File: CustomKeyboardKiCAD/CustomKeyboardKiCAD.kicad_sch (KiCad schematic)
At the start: 4 parts, among them J1 USB_C_Receptacle_USB2.0_16P, U1 nRF52840

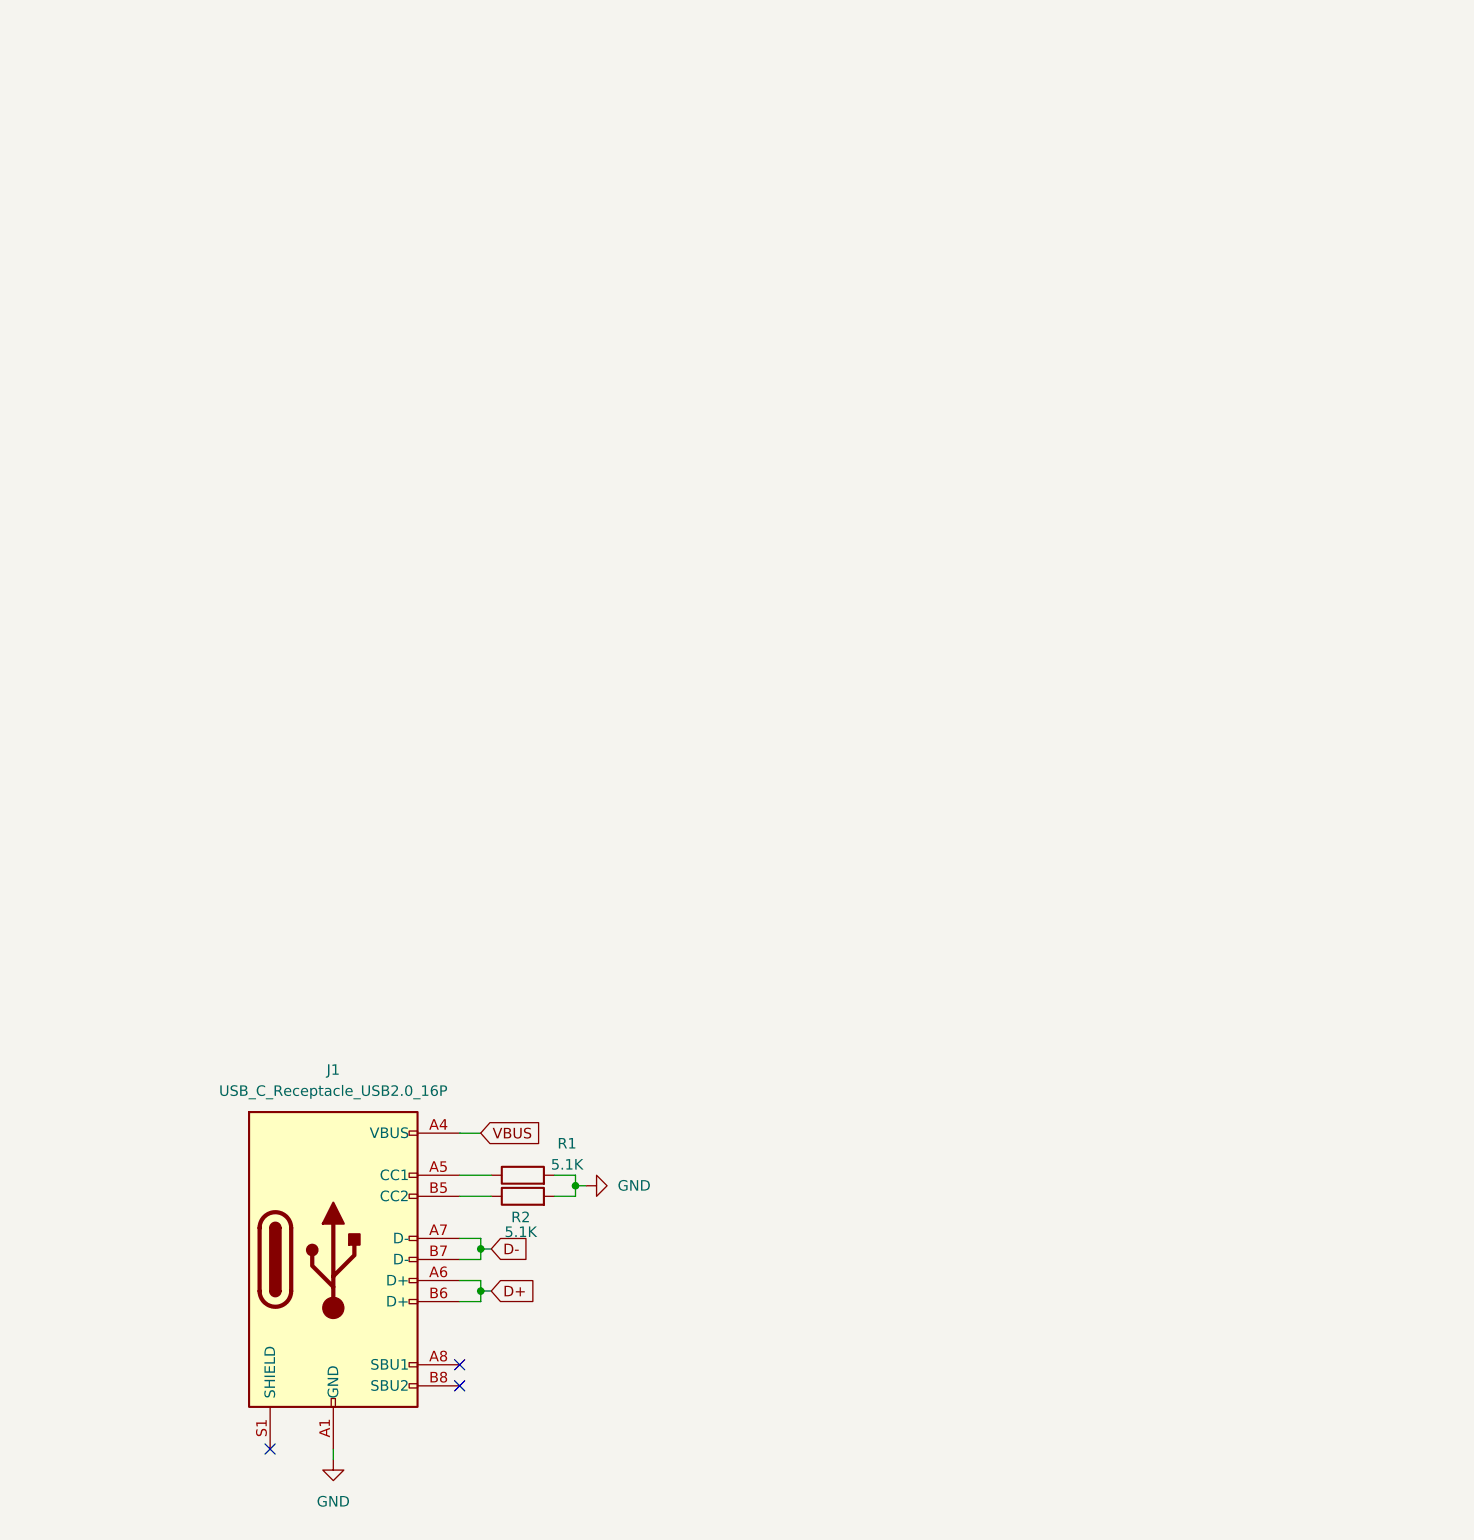
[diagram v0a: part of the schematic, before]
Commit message: Progress on schematic
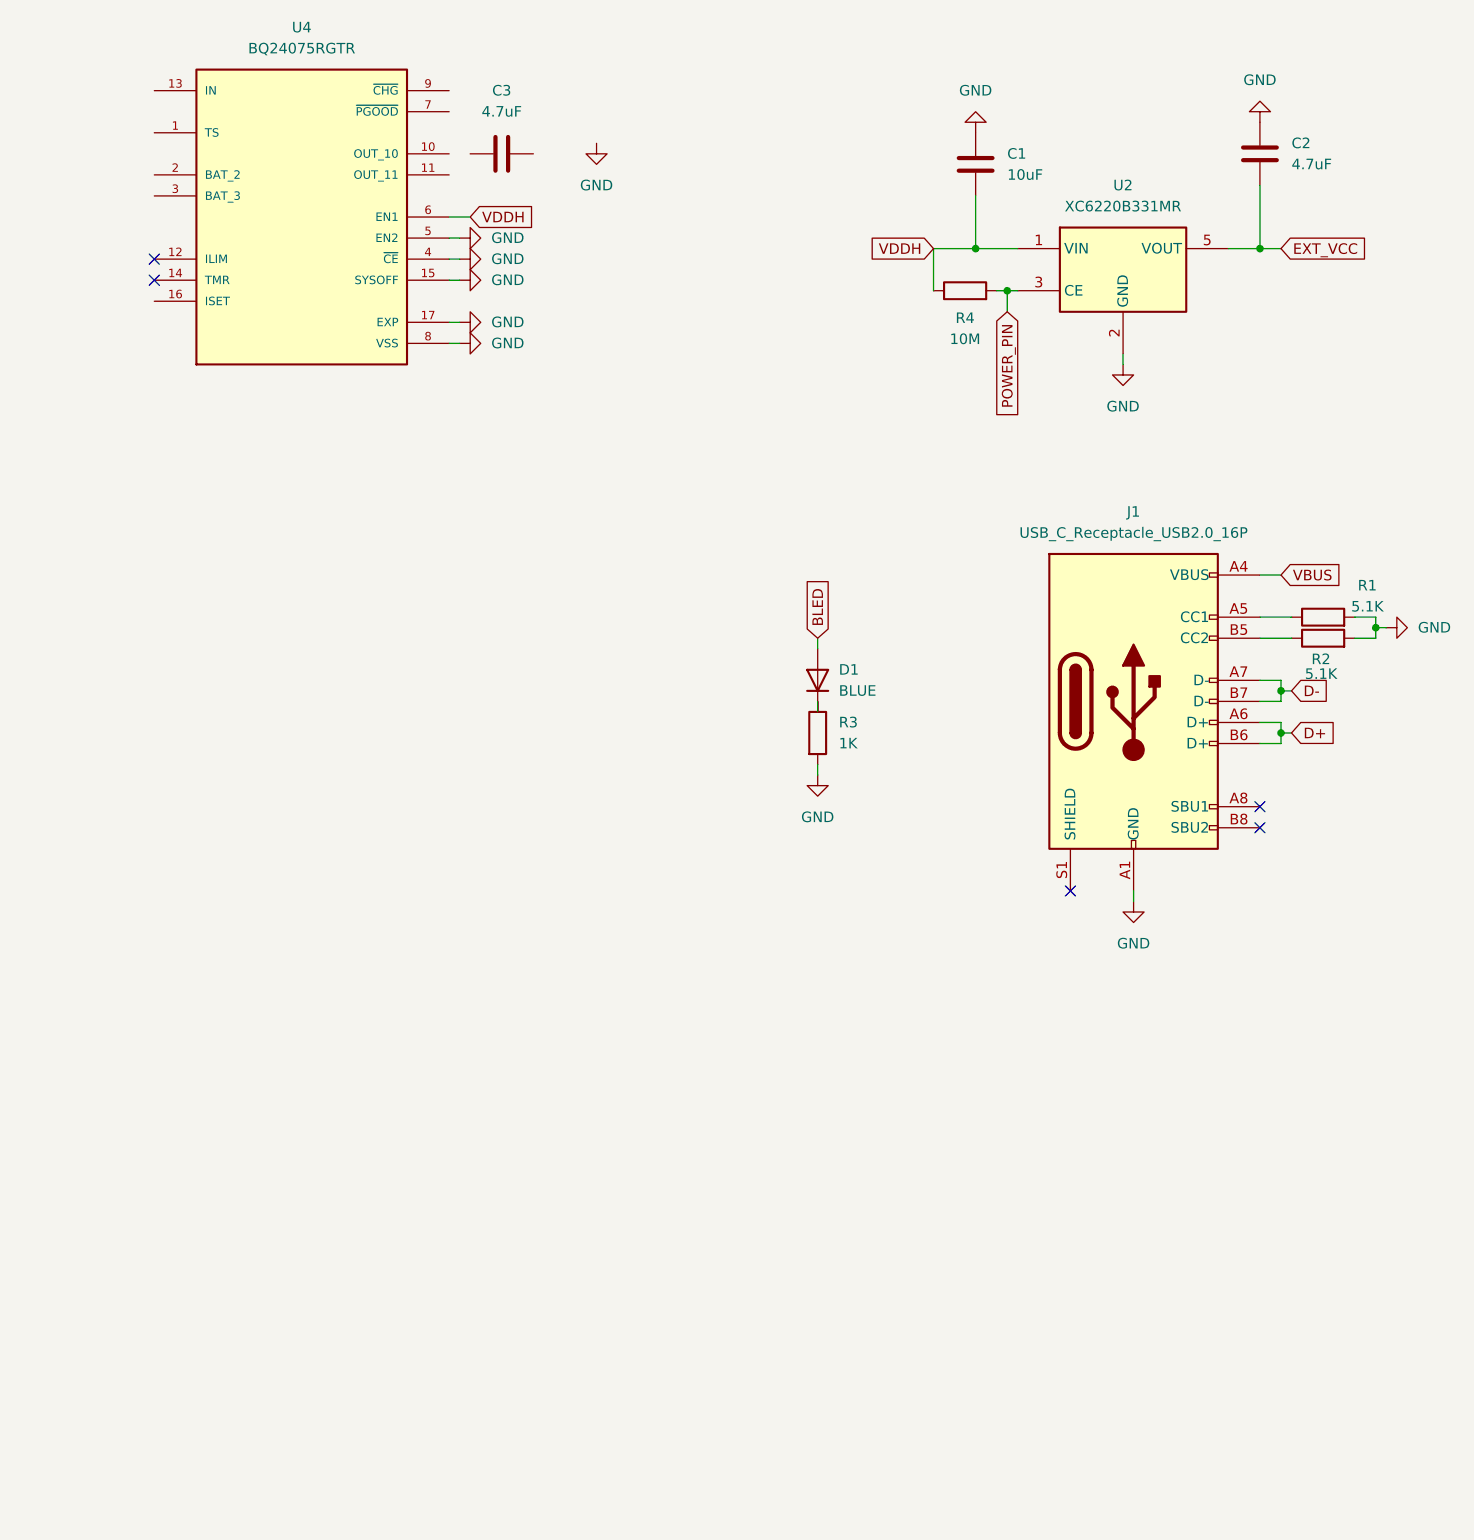
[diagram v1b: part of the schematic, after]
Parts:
- added C1: 10uF, symbol Device:C
- added C2, C3: 4.7uF, symbol Device:C
- added D1: BLUE, symbol Device:D
- added R3: 1K, symbol Device:R
- added R4: 10M, symbol Device:R
- added U2: XC6220B331MR, Package_TO_SOT_SMD:SOT-23-5, symbol Regulator_Linear:XC6220B331MR
- added U4: BQ24075RGTR, BQ24075RGTR:QFN50P300X300X100-17N, symbol BQ24075RGTR:BQ24075RGTR
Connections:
- net GND: now also C1.1, C2.1, R3.2, U2.2 (GND), U4.15 (SYSOFF), U4.17 (EXP), U4.4 (~{CE}), U4.5 (EN2), U4.8 (VSS)
- new net: D1.1 (K), R3.1
- new net BLED: D1.2 (A)
- new net EXT_VCC: C2.2, U2.5 (VOUT)
- new net POWER_PIN: R4.2, U2.3 (CE)
- new net VDDH: C1.2, R4.1, U2.1 (VIN), U4.6 (EN1)
- no-connect marks 3 -> 5
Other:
- moved on the sheet: J1, R1, R2

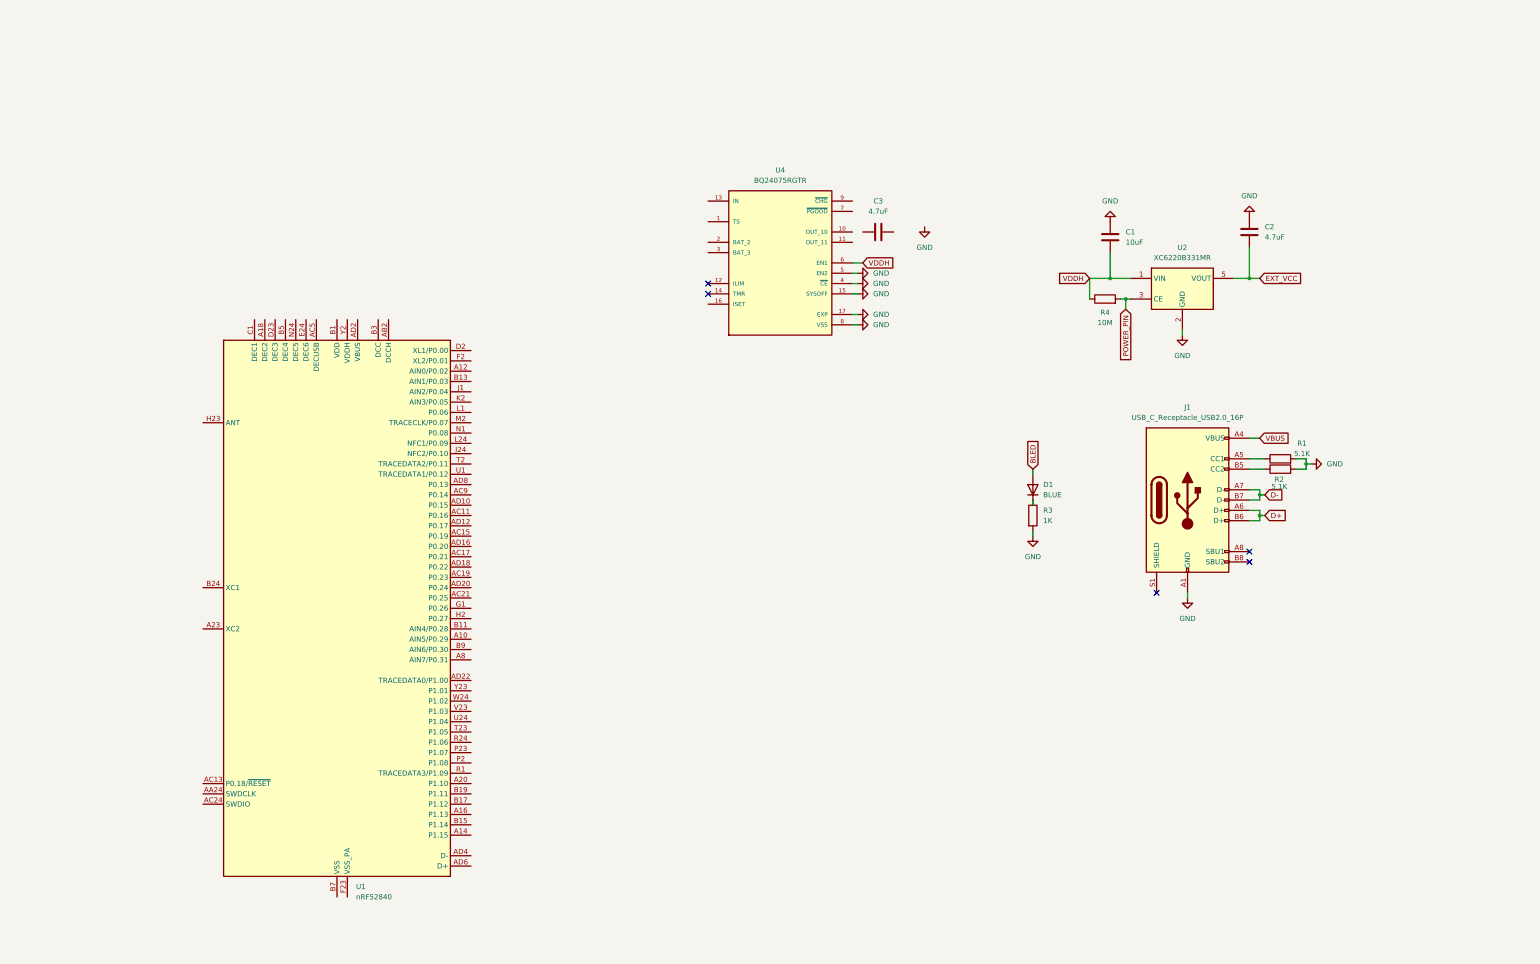
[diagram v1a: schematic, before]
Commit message: updated the schematic
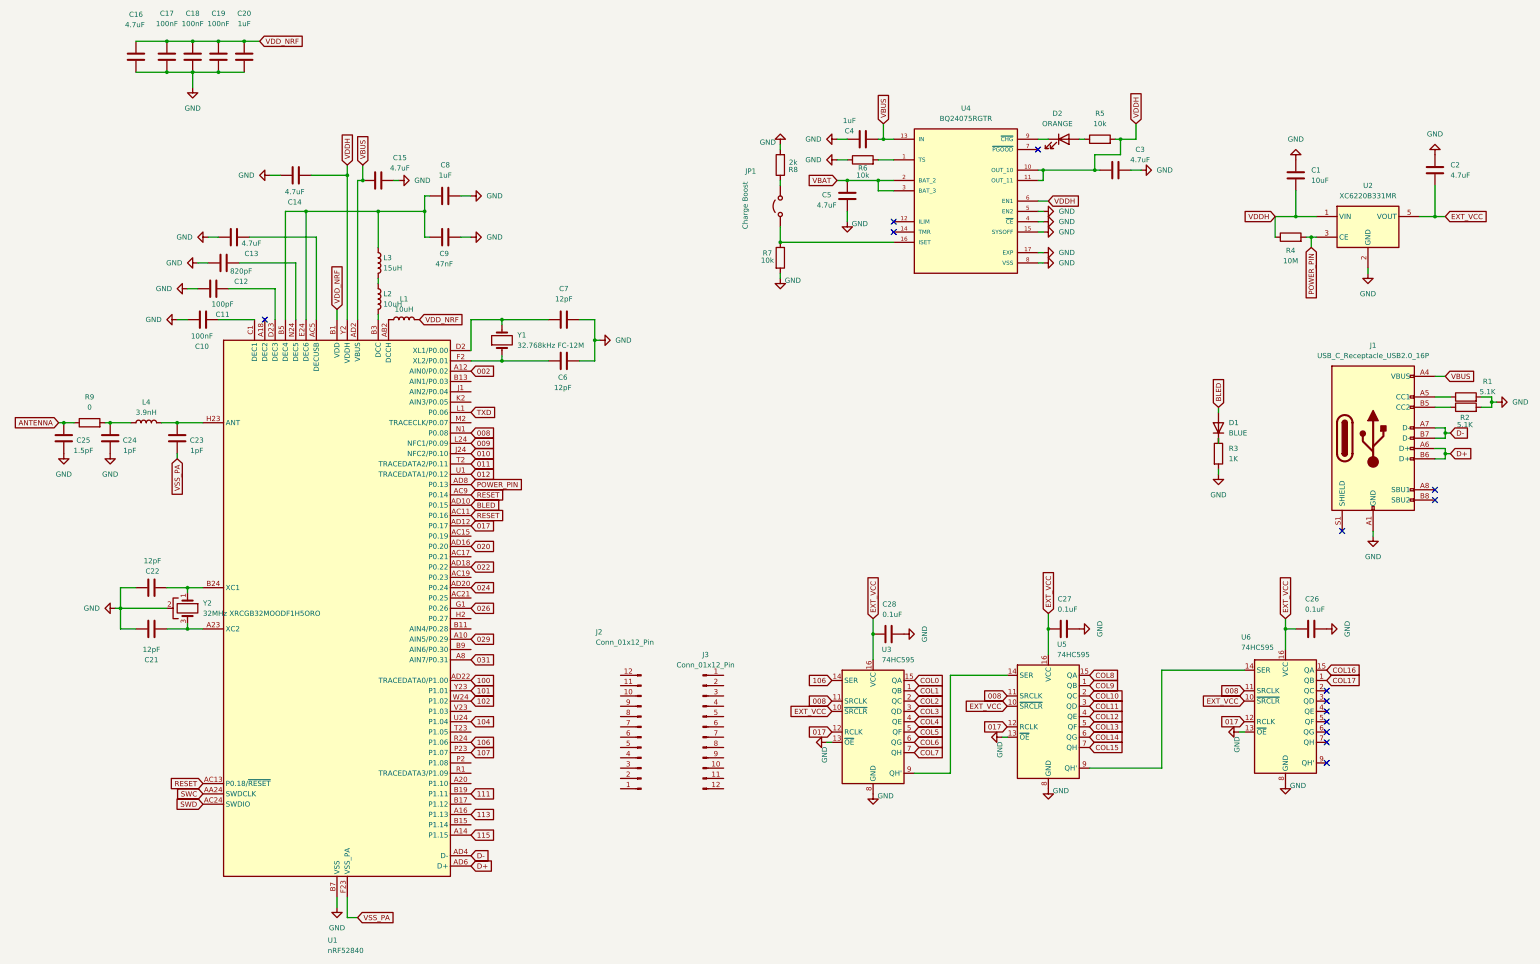
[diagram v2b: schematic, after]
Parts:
- added C10, C17, C18, C19: 100nF, symbol Device:C
- added C11: 100pF, symbol Device:C
- added C12: 820pF, symbol Device:C
- added C13, C14, C15, C16, C5: 4.7uF, symbol Device:C
- added C20, C4, C8: 1uF, symbol Device:C
- added C21, C22, C6, C7: 12pF, symbol Device:C
- added C23, C24: 1pF, symbol Device:C
- added C25: 1.5pF, symbol Device:C
- added C26, C27, C28: 0.1uF, symbol Device:C
- added C9: 47nF, symbol Device:C
- added D2: ORANGE, symbol Device:LED
- added J2, J3: Conn_01x12_Pin, symbol Connector:Conn_01x12_Pin
- added JP1: Charge Boost, symbol Jumper:Jumper_2_Open
- added L1, L2: 10uH, symbol Device:L
- added L3: 15uH, symbol Device:L
- added L4: 3.9nH, symbol Device:L
- added R5, R6, R7: 10k, symbol Device:R
- added R8: 2k, symbol Device:R
- added R9: 0, symbol Device:R
- added U3, U5, U6: 74HC595, symbol 74xx:74HC595
- added Y1: 32.768kHz FC-12M, symbol Device:Crystal
- added Y2: 32MHz XRCGB32MOODF1H5ORO, symbol Device:Crystal_GND2
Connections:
- net BLED: now also U1.AD10 (P0.15)
- net D+: now also U1.AD6 (D+)
- net D-: now also U1.AD4 (D-)
- net EXT_VCC: now also C26.2, C27.2, C28.2, U3.10 (~{SRCLR}), U3.16 (VCC), U5.10 (~{SRCLR}), U5.16 (VCC), U6.10 (~{SRCLR}), U6.16 (VCC)
- net GND: now also C3.2, U1.B7 (VSS), U1.EP (VSS), C10.2, C11.2, C12.2, C13.2, C14.2, C15.2, C16.2, C17.2, C18.2, C19.2, C20.2, C21.2, C22.2, C24.2, C25.2, C26.1, C27.1, C28.1, C4.2, C5.2, C6.2, C7.2, C8.2, C9.2, R6.1, R7.2, R8.2, U3.13 (~{OE}), U3.8 (GND), U5.13 (~{OE}), U5.8 (GND), U6.13 (~{OE}), U6.8 (GND), Y2.2
- net POWER_PIN: now also U1.AD8 (P0.13)
- net VBUS: now also U1.AD2 (VBUS), U4.13 (IN), C15.1, C4.1
- net VDDH: now also C3.1, U1.Y2 (VDDH), U4.10 (OUT_10), U4.11 (OUT_11), C14.1, R5.2
- net 029: now reaches U1.A10 (AIN5/P0.29)
- net 002: now reaches U1.A12 (AIN0/P0.02)
- net 115: now reaches U1.A14 (P1.15)
- net 113: now reaches U1.A16 (P1.13)
- net VDD_NRF: now reaches U1.A22 (VDD), U1.AD14 (VDD), U1.AD23 (VDD), U1.B1 (VDD), U1.W1 (VDD)
- net VDD_NRF: now also C16.1, C17.1, C18.1, C19.1, C20.1, L1.2
- net at U1.A23 (XC2): now also C21.1, Y2.3
- net 031: now reaches U1.A8 (AIN7/P0.31)
- net SWC: now reaches U1.AA24 (SWDCLK)
- net at U1.AB2 (DCCH): now also L1.1
- net RESET: now reaches U1.AC11 (P0.16)
- net RESET: now also U1.AC13 (P0.18/~{RESET}), U1.AC9 (P0.14)
- net SWD: now reaches U1.AC24 (SWDIO)
- net at U1.AC5 (DECUSB): now also C13.1
- net 017: now reaches U1.AD12 (P0.17)
- net 017: now also U3.12 (RCLK), U5.12 (RCLK), U6.12 (RCLK)
- net 020: now reaches U1.AD16 (P0.20)
- net 022: now reaches U1.AD18 (P0.22)
- net 024: now reaches U1.AD20 (P0.24)
- net 100: now reaches U1.AD22 (TRACEDATA0/P1.00)
- net 111: now reaches U1.B19 (P1.11)
- net at U1.B24 (XC1): now also C22.1, Y2.1
- net at U1.B3 (DCC): now also L2.2
- net at U1.B5 (DEC4): now also U1.E24 (DEC6), C8.1, C9.1, L3.1
- net at U1.C1 (DEC1): now also C10.1
- net at U1.D2 (XL1/P0.00): now also C7.1, Y1.2
- net at U1.D23 (DEC3): now also C11.1
- net at U1.F2 (XL2/P0.01): now also C6.1, Y1.1
- net VSS_PA: now reaches U1.F23 (VSS_PA)
- net VSS_PA: now also C23.2
- net 026: now reaches U1.G1 (P0.26)
- net at U1.H23 (ANT): now also C23.1, L4.2
- net 010: now reaches U1.J24 (NFC2/P0.10)
- net TXD: now reaches U1.L1 (P0.06)
- net 009: now reaches U1.L24 (NFC1/P0.09)
- net 008: now reaches U1.N1 (P0.08)
- net 008: now also U3.11 (SRCLK), U5.11 (SRCLK), U6.11 (SRCLK)
- net at U1.N24 (DEC5): now also C12.1
- net 107: now reaches U1.P23 (P1.07)
- net 106: now reaches U1.R24 (P1.06)
- net 106: now also U3.14 (SER)
- net 011: now reaches U1.T2 (TRACEDATA2/P0.11)
- net 012: now reaches U1.U1 (TRACEDATA1/P0.12)
- net 104: now reaches U1.U24 (P1.04)
- net 102: now reaches U1.W24 (P1.02)
- net 101: now reaches U1.Y23 (P1.01)
- net at U4.1 (TS): now also R6.2
- net at U4.16 (ISET): now also JP1.1 (A), R7.1
- net VBAT: now reaches U4.2 (BAT_2)
- net VBAT: now also U4.3 (BAT_3), C5.1
- net at U4.9 (~{CHG}): now also D2.1 (K)
- new net: D2.2 (A), R5.1
- new net: JP1.2 (B), R8.1
- new net: U3.9 (QH'), U5.14 (SER)
- new net: U5.9 (QH'), U6.14 (SER)
- new net: L2.1, L3.2
- new net: C24.1, L4.1, R9.2
- new net ANTENNA: C25.1, R9.1
- new net COL0: U3.15 (QA)
- new net COL1: U3.1 (QB)
- new net COL10: U5.2 (QC)
- new net COL11: U5.3 (QD)
- new net COL12: U5.4 (QE)
- new net COL13: U5.5 (QF)
- new net COL14: U5.6 (QG)
- new net COL15: U5.7 (QH)
- new net COL16: U6.15 (QA)
- new net COL17: U6.1 (QB)
- new net COL2: U3.2 (QC)
- new net COL3: U3.3 (QD)
- new net COL4: U3.4 (QE)
- new net COL5: U3.5 (QF)
- new net COL6: U3.6 (QG)
- new net COL7: U3.7 (QH)
- new net COL8: U5.15 (QA)
- new net COL9: U5.1 (QB)
- no-connect marks 5 -> 14
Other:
- moved on the sheet: C1, C2, C3, D1, J1, R1, R2, R3, R4, U2, U4
